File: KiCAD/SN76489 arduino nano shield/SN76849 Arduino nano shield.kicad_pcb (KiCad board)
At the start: 2 copper layers, 73.8 x 53 mm, 14 parts, among them J1 Arduino_in, J2 audio_debug, J3 OLED_wit, J5 LOGO, J6 gat1, J7 gat2, J8 geluid_uit, U1 PCF8574, U3 SN76489, X1 CLK_DIP14_4Mhz

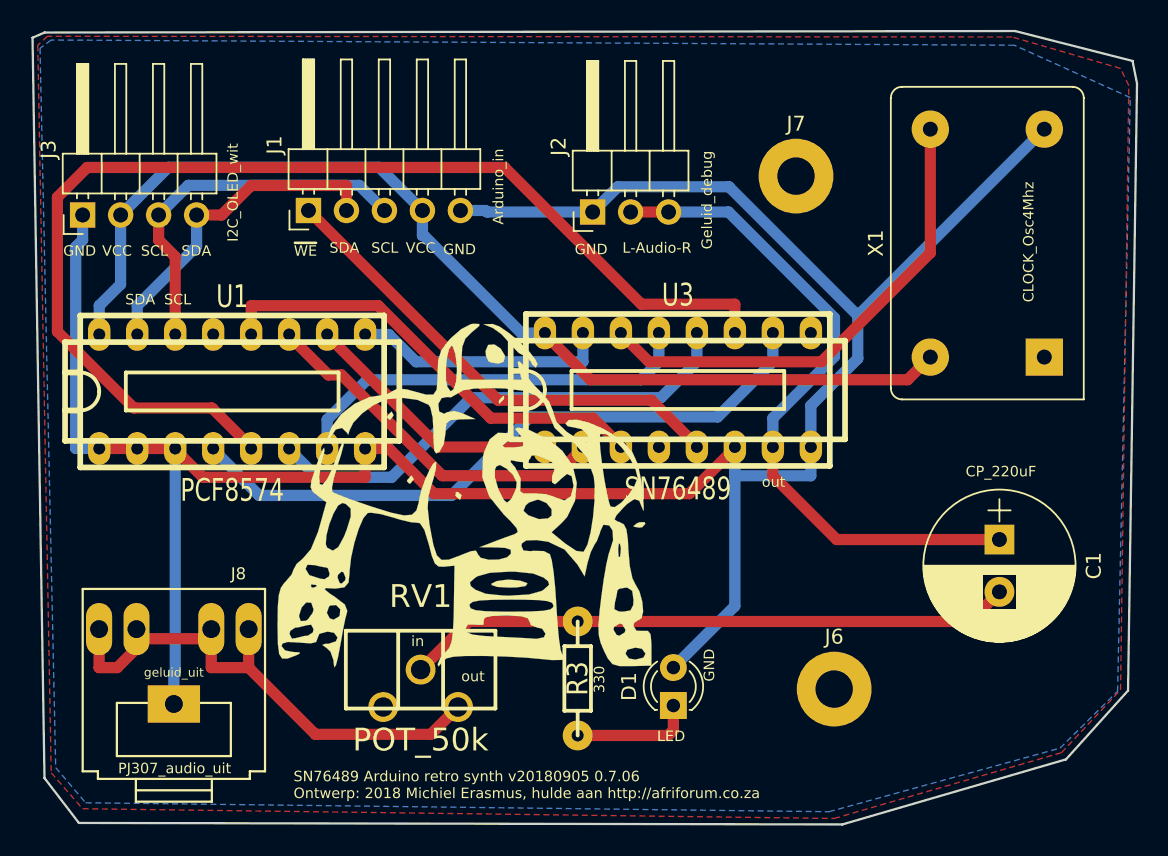
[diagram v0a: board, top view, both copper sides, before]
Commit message: versie 20180905 0.7.06
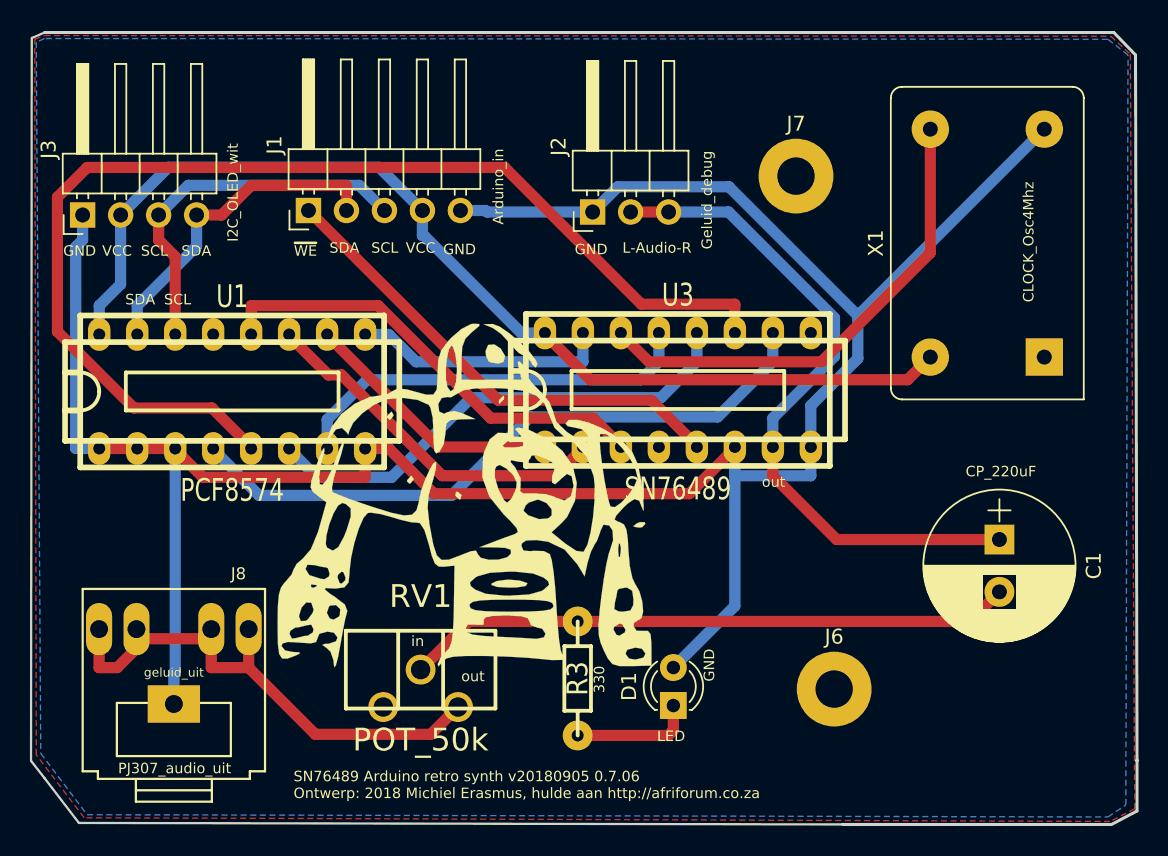
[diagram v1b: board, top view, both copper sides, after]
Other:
- board size 73.8 x 53 mm -> 74 x 52.9 mm
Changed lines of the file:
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@@
   (general
     (thickness 1.6)
-    (drawings 36)
+    (drawings 38)
     (tracks 150)
     (zones 0)
@@
     )
   )
+  (gr_line (start 34.25 71.3) (end 34.25 71.6) (layer Edge.Cuts) (width 0.15))
+  (gr_line (start 35.15 72.75) (end 34.25 71.6) (layer Edge.Cuts) (width 0.15))
+  (gr_line (start 34.3 23.25) (end 34.25 71.3) (layer Edge.Cuts) (width 0.15))
+  (gr_line (start 106.5 75.85) (end 108.2 74.95) (layer Edge.Cuts) (width 0.2))
+  (gr_line (start 108.2 71.55) (end 108.2 74.95) (layer Edge.Cuts) (width 0.2))
+  (gr_line (start 88.5 75.85) (end 106.45 75.85) (layer Edge.Cuts) (width 0.2))
+  (gr_line (start 108.1 24.4) (end 108.2 71.6) (layer Edge.Cuts) (width 0.2))
+  (gr_line (start 106.65 22.9) (end 108.1 24.4) (layer Edge.Cuts) (width 0.2))
+  (gr_line (start 35.15 22.9) (end 106.65 22.9) (layer Edge.Cuts) (width 0.2))
   (gr_line (start 34.35 23.25) (end 35.15 22.9) (layer Edge.Cuts) (width 0.15))
-  (gr_line (start 35.15 72.75) (end 34.35 23.25) (layer Edge.Cuts) (width 0.15))
   (gr_line (start 37.45 75.75) (end 35.15 72.75) (layer Edge.Cuts) (width 0.15))
   (gr_line (start 88.5 75.85) (end 37.45 75.75) (layer Edge.Cuts) (width 0.15))
-  (gr_line (start 103.45 71.5) (end 88.5 75.85) (layer Edge.Cuts) (width 0.15))
-  (gr_line (start 107.6 66.9) (end 103.45 71.5) (layer Edge.Cuts) (width 0.15))
-  (gr_line (start 108.2 26.3) (end 107.6 66.9) (layer Edge.Cuts) (width 0.15))
-  (gr_line (start 107.9 24.8) (end 108.2 26.3) (layer Edge.Cuts) (width 0.15))
-  (gr_line (start 100.05 22.8) (end 107.9 24.8) (layer Edge.Cuts) (width 0.15))
-  (gr_line (start 35.15 22.9) (end 100.05 22.8) (layer Edge.Cuts) (width 0.15))
   (gr_text 330 (at 72.25 66.15 90) (layer F.SilkS)
     (effects (font (size 0.7 0.7) (thickness 0.175)))
@@
     (polygon
       (pts
-        (xy 34.7 23.75) (xy 35.6 72.4) (xy 37.7 74.8) (xy 87.95 75.45) (xy 103.15 71.05)
-        (xy 107.1 66.85) (xy 107.65 26.45) (xy 107.1 25.3) (xy 99.85 23.2) (xy 35.35 23.15)
+        (xy 108.05 74.8) (xy 106.4 75.65) (xy 37.8 75.4) (xy 34.6 71.2) (xy 34.5 23.35)
+        (xy 35.15 23.1) (xy 106.45 23.15) (xy 107.75 24.35)
       )
     )
@@
     (polygon
       (pts
-        (xy 34.85 23.95) (xy 35.9 72.05) (xy 37.9 74.4) (xy 87.6 75) (xy 103.05 70.75)
-        (xy 106.9 66.95) (xy 107.75 27.25) (xy 100 23.75) (xy 35.6 23.4)
+        (xy 106.25 23.35) (xy 35.15 23.3) (xy 34.6 23.55) (xy 34.9 71.1) (xy 38 75.2)
+        (xy 106.25 75.35) (xy 107.45 74.55) (xy 107.6 24.4)
       )
     )
